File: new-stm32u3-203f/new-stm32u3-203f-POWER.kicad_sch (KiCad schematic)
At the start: 30 parts, among them J4 Battery connector, SW2 SW_SPDT, U4 LD39050PU33R, U5 TLV62569DBVR, U6 MCP73831T-2ACI/OT, U7 TPS63802DLAR

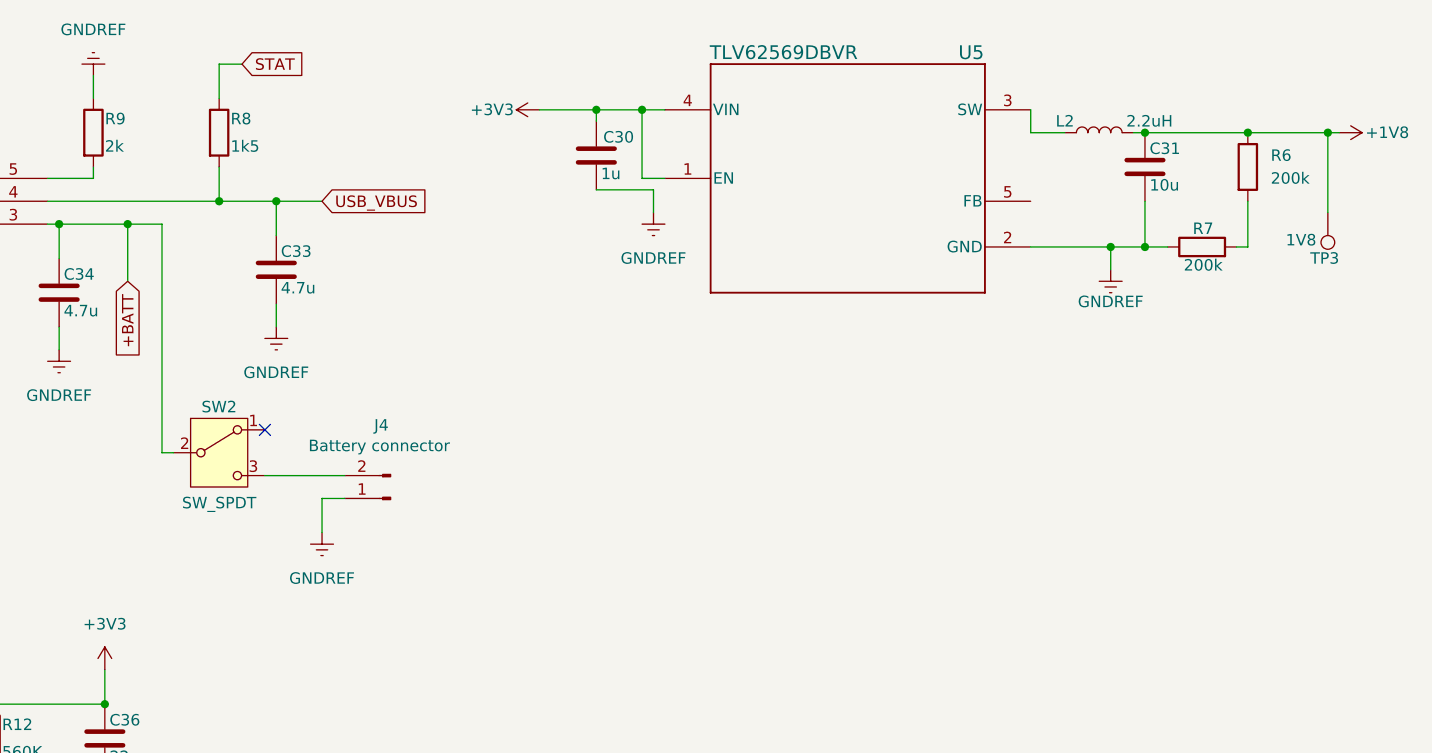
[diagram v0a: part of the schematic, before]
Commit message: finished the schematic, just need someone to review it :)
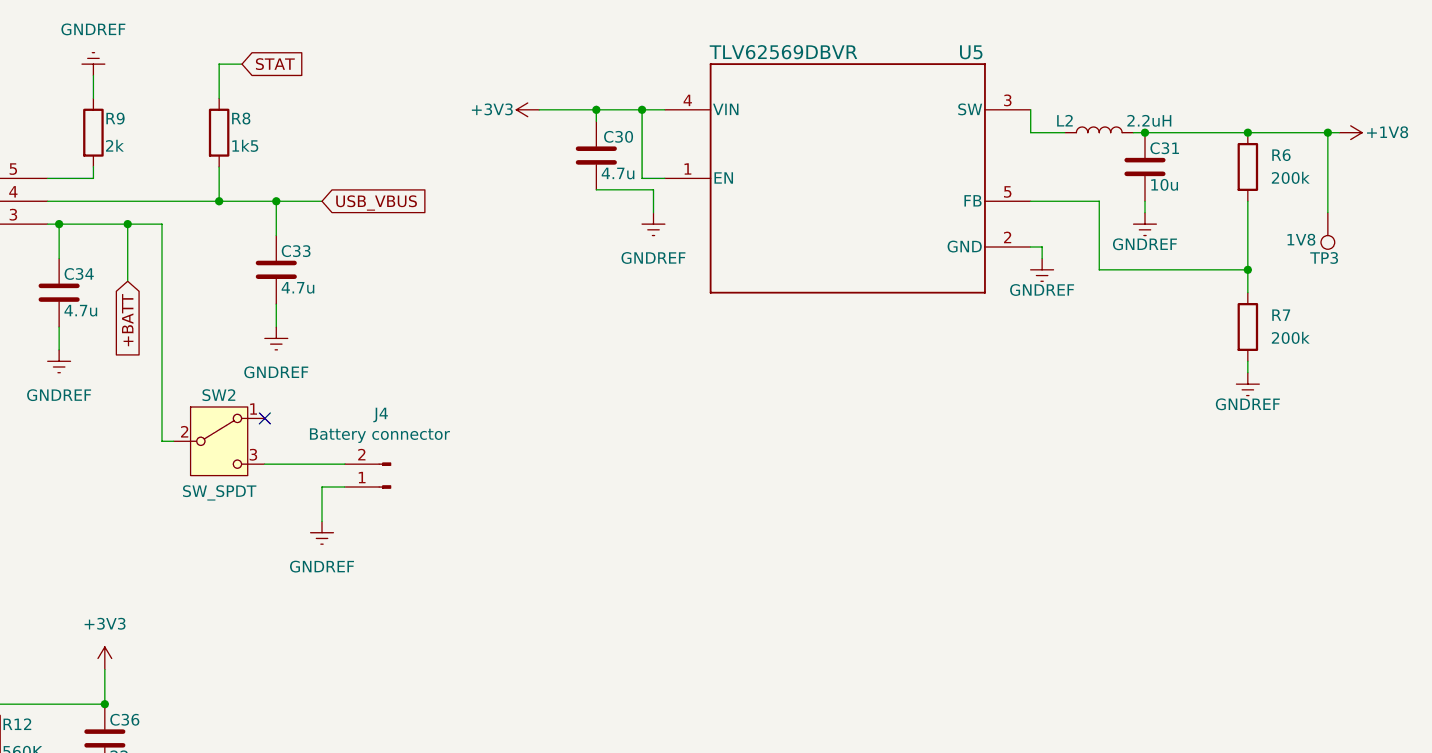
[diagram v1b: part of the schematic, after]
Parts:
- C30: value 1u -> 4.7u
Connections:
- net GNDREF: now also R7.2; no longer R7.1
- net at R6.2: now also R7.1, U5.5 (FB); no longer R7.2
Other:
- moved on the sheet: J4, SW2
